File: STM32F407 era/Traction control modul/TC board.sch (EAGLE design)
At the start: 10 parts, among them IC1 TL072D

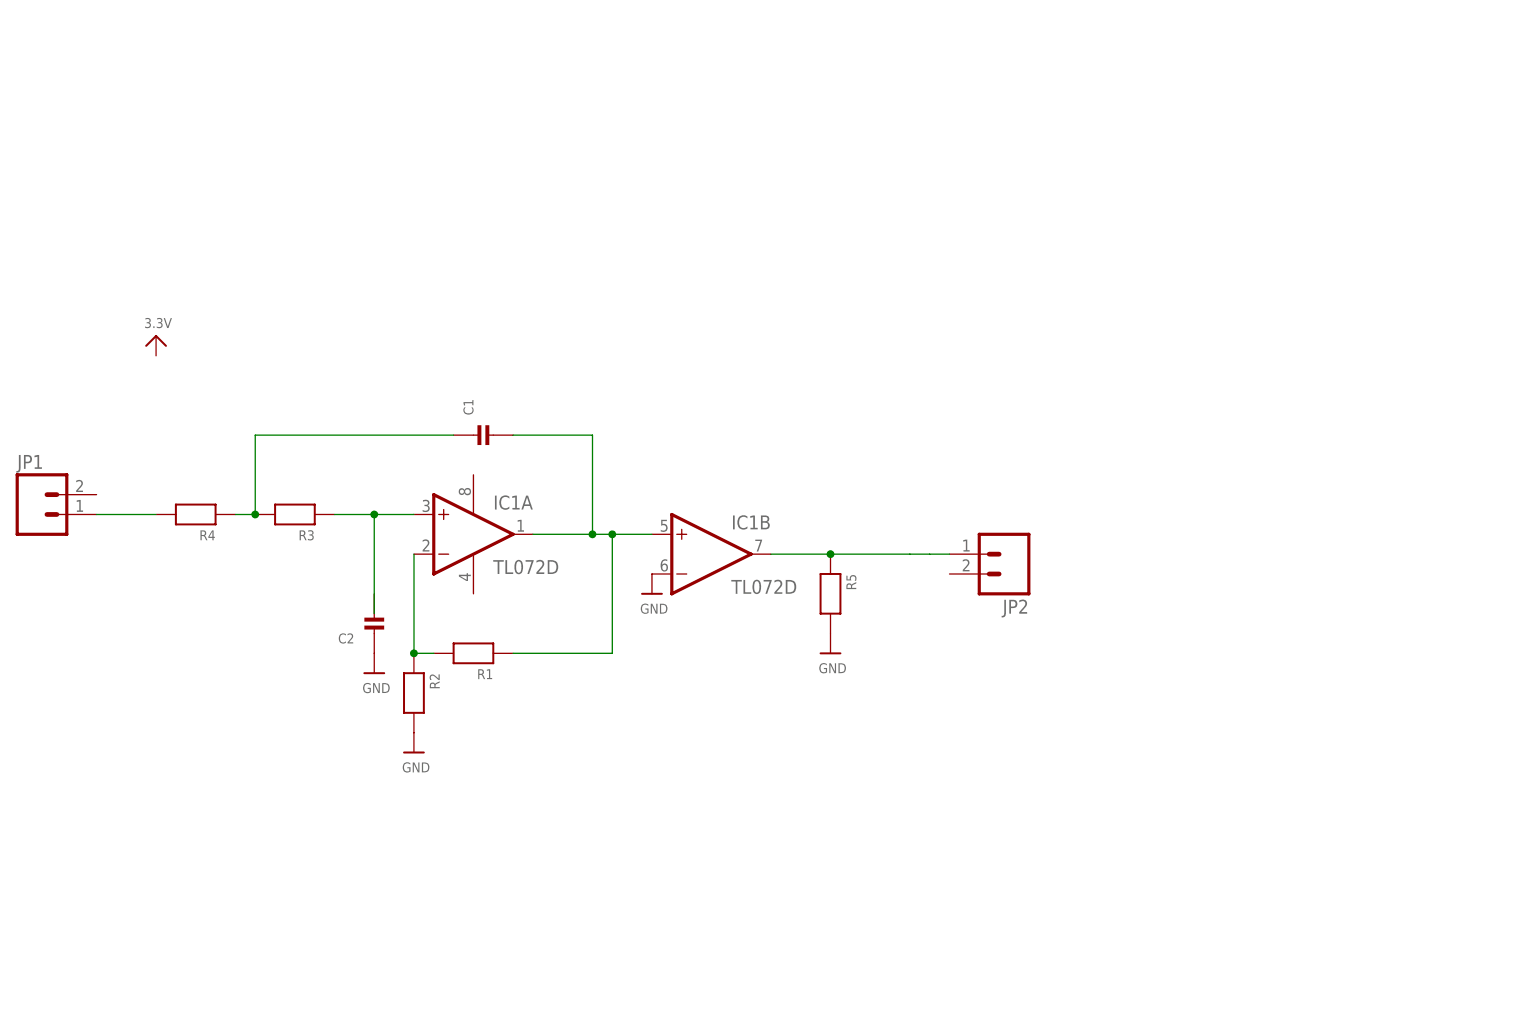
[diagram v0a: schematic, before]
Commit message: started work on traction control node
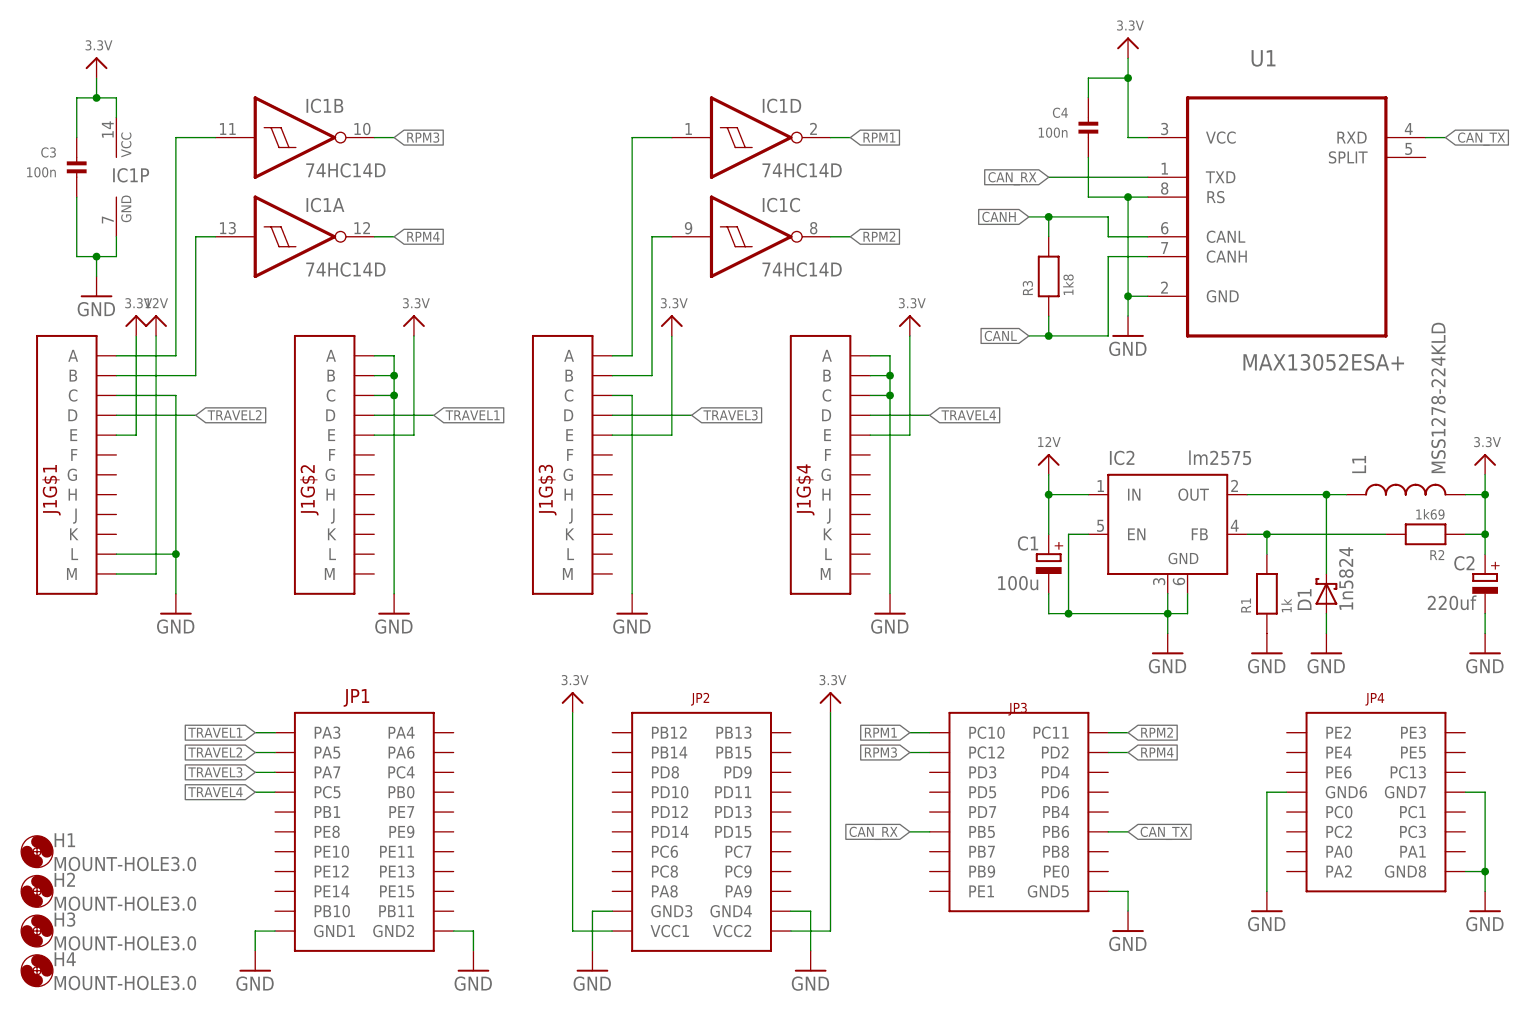
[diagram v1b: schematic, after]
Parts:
- removed JP1, JP2: (no value), unicorn_v2:M02-JST-2MM-SMT
- removed R4, R5: (no value), microbuilder:RESISTOR0603
- added C3, C4: 100n, microbuilder:CAP_CERAMIC_0603
- added D1: 1n5824, diode:SCHOTTKY-DIODEF126Z12
- added H1, H2, H3, H4: MOUNT-HOLE3.0, holes:MOUNT-HOLE3.0
- added IC2: lm2575, linear:LM2596S
- added J1: (no value), unicorn_v2:AUTOCONNECTOR
- added L1: MSS1278-224KLD, SparkFun-Passives:INDUCTORPWR
- added U$1: CPU-BOARD, unicorn_v2:CPU-BOARD
- added U1: MAX13052ESA+, Maxim_By_element14_Batch_1:MAX13052ESA+
- C1: value (none) -> 100u; device microbuilder:CAP_CERAMIC0603 -> rcl:CPOL-EUE2.5-7
- C2: value (none) -> 220uf; device microbuilder:CAP_CERAMIC0603 -> rcl:CPOL-EUE3.5-8
- IC1: value TL072D -> 74HC14D; device linear:TL072D -> 74xx-eu:74HC14D
- R1: value (none) -> 1k; device microbuilder:RESISTOR0603 -> microbuilder:RESISTOR_0603
- R2: value (none) -> 1k69; device microbuilder:RESISTOR0603 -> microbuilder:RESISTOR_0603
- R3: value (none) -> 1k8; device microbuilder:RESISTOR0603 -> microbuilder:RESISTOR_0603
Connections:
- removed net N$7: IC1B.OUT, JP2.1, R5.1
- new net 12V: C1.+, IC2.IN, J1G$1.M
- new net 3.3V: C2.+, C3.P$1, C4.P$1, IC1P.VCC, J1G$1.E, J1G$2.E, J1G$3.E, J1G$4.E, L1.2, R2.1, U$1G$2.VCC1, U$1G$2.VCC2, U1.VCC
- new net CANH: R3.2, U1.CANL
- new net CANL: R3.1, U1.CANH
- new net CAN_RX: U$1G$3.PB5, U1.TXD
- new net CAN_TX: U$1G$3.PB6, U1.RXD
- new net N$6: IC1C.I, J1G$3.B
- new net RPM1: IC1D.O, U$1G$3.PC10
- new net RPM2: IC1C.O, U$1G$3.PC11
- new net RPM3: IC1B.O, U$1G$3.PC12
- new net RPM4: IC1A.O, U$1G$3.PD2
- new net TRAVEL1: J1G$2.D, U$1G$1.PA3
- new net TRAVEL2: J1G$1.D, U$1G$1.PA5
- new net TRAVEL3: J1G$3.D, U$1G$1.PA7
- new net TRAVEL4: J1G$4.D, U$1G$1.PC5
- net GND: now also C1.-, C2.-, C3.P$2, C4.P$2, D1.A, IC1P.GND, IC2.EN, IC2.GND, IC2.GND@1, J1G$1.C, J1G$1.L, J1G$2.A, J1G$2.B, J1G$2.C, J1G$3.C, J1G$4.A, J1G$4.B, J1G$4.C, R1.1, U$1G$1.GND1, U$1G$1.GND2, U$1G$2.GND3, U$1G$2.GND4, U$1G$3.GND5, U$1G$4.GND6, U$1G$4.GND7, U$1G$4.GND8, U1.GND, U1.RS; no longer C2.P$1, IC1B.-IN, R2.2, R5.2
- net N$1: now also IC2.FB, R1.2, R2.2; no longer JP1.1, R4.2
- net N$2: now also D1.C, IC2.OUT, L1.1; no longer C1.P$1, R3.2, R4.1
- net N$3: now also IC1B.I, J1G$1.A; no longer IC1A.+IN, R3.1
- net N$4: now also IC1A.I, J1G$1.B; no longer C1.P$2, IC1A.OUT, IC1B.+IN, R1.1
- net N$5: now also IC1D.I, J1G$3.A; no longer IC1A.-IN, R1.2, R2.1
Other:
- moved on the sheet: R1, R2, R3
